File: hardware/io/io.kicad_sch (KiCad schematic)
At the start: 784 parts, among them J1 USB_B, J10 Conn_02x18_Odd_Even, J11 Barrel_Jack_Switch_Pin3Ring, J2 Conn_02x03_Odd_Even, J3 Conn_02x08_Odd_Even, J4 Conn_02x40_Odd_Even, J5 Conn_02x16_Odd_Even, J6 Conn_02x16_Odd_Even, J7 Conn_02x12_Odd_Even, J8 Conn_02x24_Odd_Even, Q129 IRLML6244, Q130 IRLML6402, Q131 IRLML6244, Q132 IRLML6402, Q133 IRLML6244, Q134 IRLML6402, Q135 IRLML6244, Q136 IRLML6402, Q137 IRLML6244, Q138 IRLML6402, Q139 IRLML6244, Q140 IRLML6402, Q141 IRLML6244, Q142 IRLML6402, Q143 IRLML6244, Q144 IRLML6402, Q145 IRLML6244, Q146 IRLML6402, Q147 IRLML6244, Q148 IRLML6402, Q149 IRLML6244, Q150 IRLML6402, Q151 IRLML6244, Q152 IRLML6402, Q153 IRLML6244, Q154 IRLML6402, Q155 IRLML6244, Q156 IRLML6402, Q157 IRLML6244, Q158 IRLML6402, Q159 IRLML6244, Q160 IRLML6402, Q161 IRLML6244, Q162 IRLML6402, Q163 IRLML6244, Q164 IRLML6402, Q165 IRLML6244, Q166 IRLML6402, Q167 IRLML6244, Q168 IRLML6402, Q169 IRLML6244, Q170 IRLML6402, Q171 IRLML6244, Q172 IRLML6402, Q173 IRLML6244, Q174 IRLML6402, Q175 IRLML6244, Q176 IRLML6402, Q177 IRLML6244, Q178 IRLML6402, Q179 IRLML6244, Q180 IRLML6402, Q181 IRLML6244, Q182 IRLML6402, Q183 IRLML6244, Q184 IRLML6402, Q185 IRLML6244, Q186 IRLML6402, Q187 IRLML6244, Q188 IRLML6402, Q189 IRLML6244, Q190 IRLML6402, Q191 IRLML6244, Q192 IRLML6402, Q193 IRLML6244, Q194 IRLML6402, Q195 IRLML6244, Q196 IRLML6402, Q197 IRLML6244, Q198 IRLML6402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

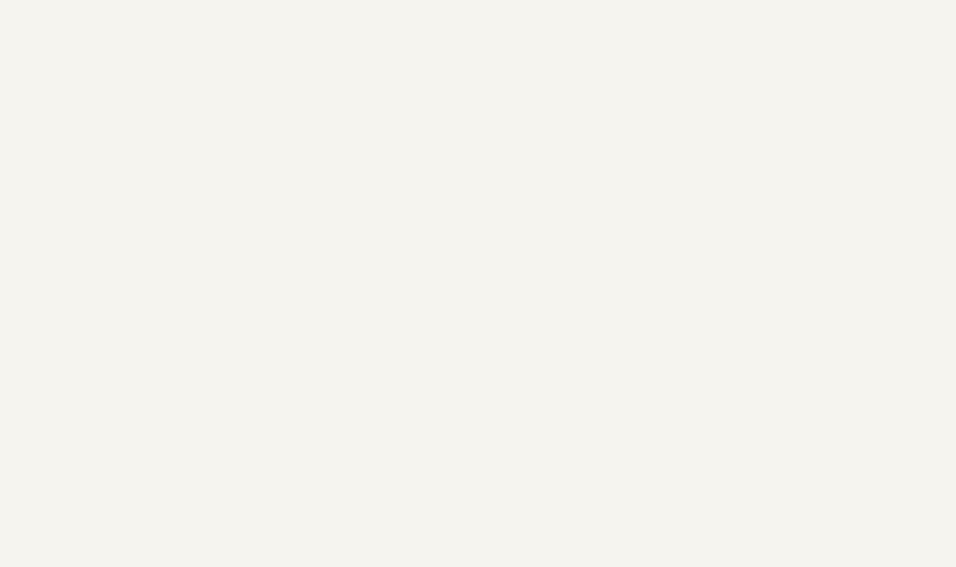
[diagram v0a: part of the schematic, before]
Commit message: io pcb done. :)
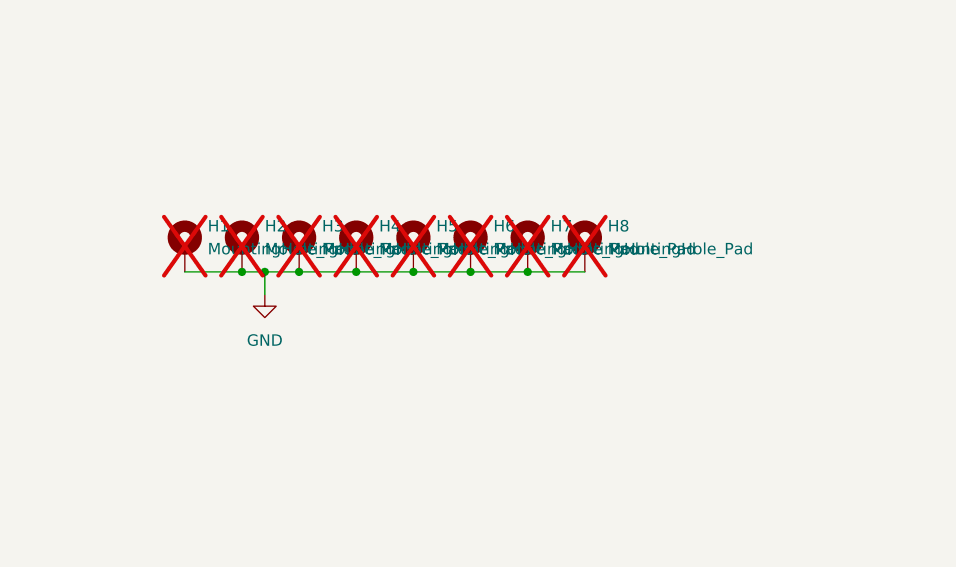
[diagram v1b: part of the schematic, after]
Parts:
- added H1, H2, H3, H4, H5, H6, H7, H8: MountingHole_Pad, MountingHole:MountingHole_3.2mm_M3_ISO7380_Pad_TopBottom, symbol Mechanical:MountingHole_Pad
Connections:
- net GND: now also H1.1, H2.1, H3.1, H4.1, H5.1, H6.1, H7.1, H8.1
